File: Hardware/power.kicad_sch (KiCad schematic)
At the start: 16 parts, among them U1 TPS7A20L_1V2, U4 TPS7A20L_2V2, U6 TPS7A20L_3V3, U7 ICE40UL1K-CM36AI

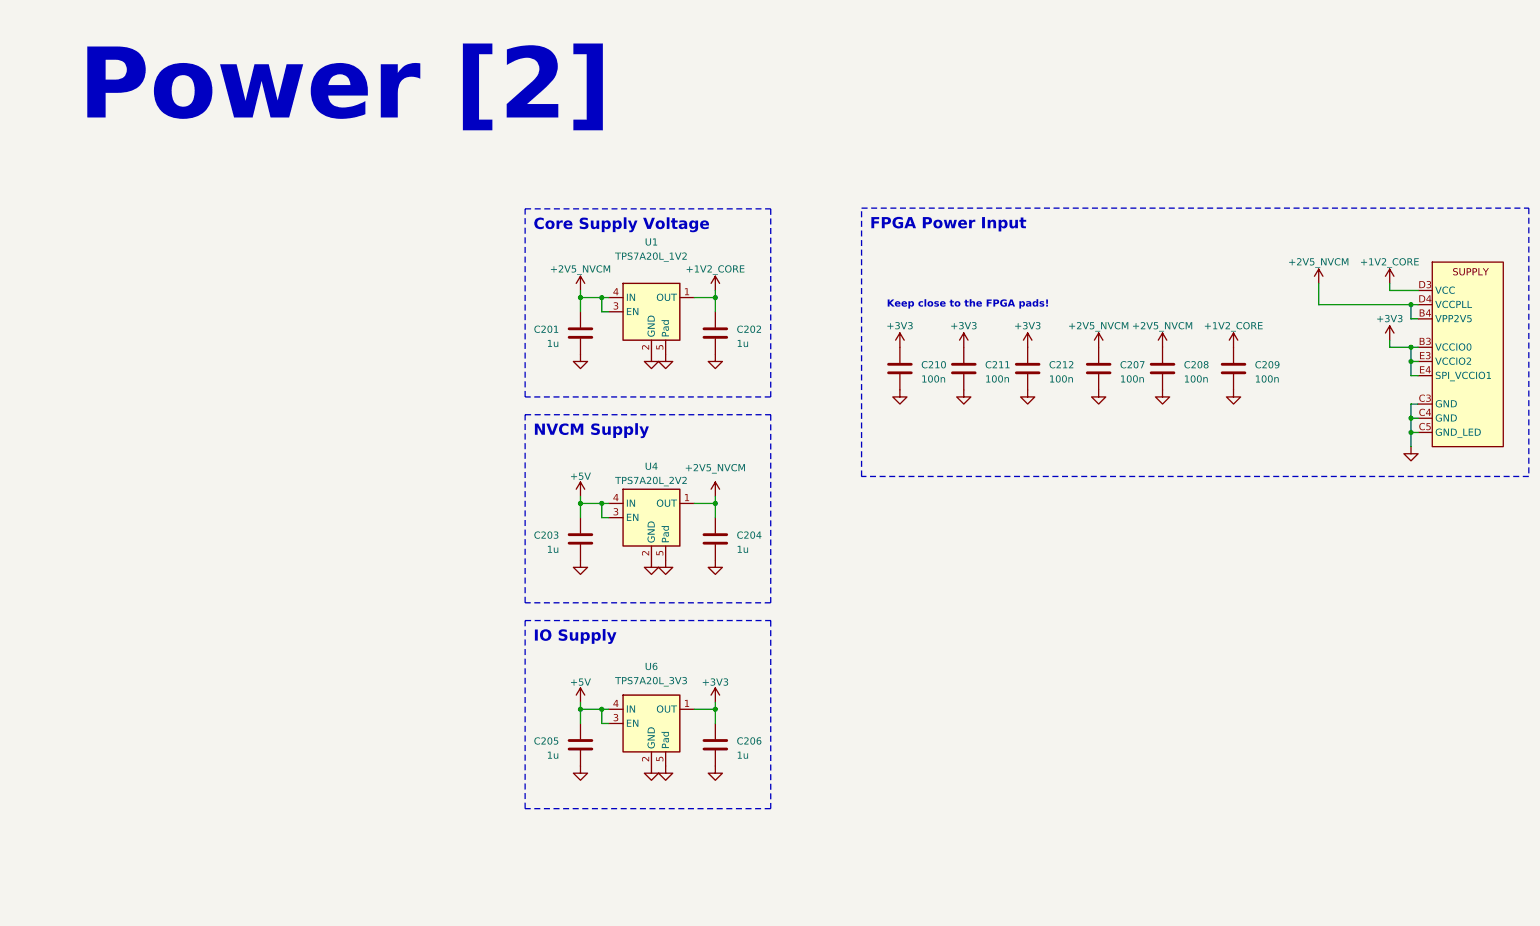
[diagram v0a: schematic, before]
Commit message: Added schematic sections and advanced the design. Advanced the development of Verilog code, for TinyFPGA bringup (however, still not working). Cosmetic changes in README.
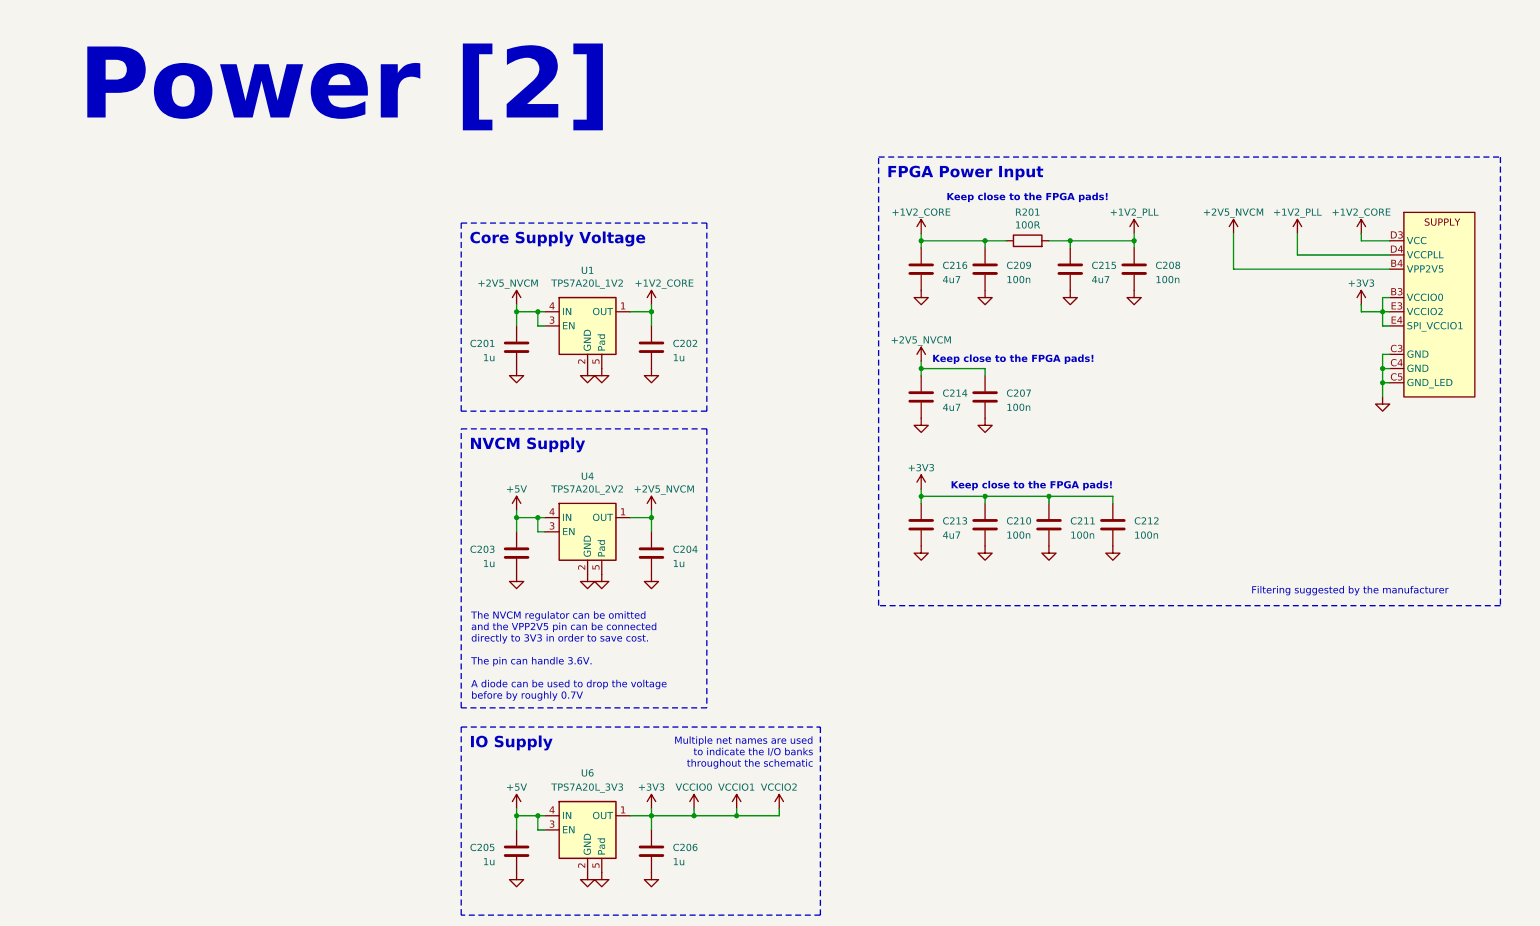
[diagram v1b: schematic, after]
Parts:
- added C213, C214, C215, C216: 4u7, symbol Device:C
- added R201: 100R, symbol Device:R
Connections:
- net +1V2_CORE: now also C216.1, R201.1
- net +2V5_NVCM: now also C214.1; no longer C208.1, U7.D4 (VCCPLL)
- net +3V3: now also C213.1
- net GND: now also C213.2, C214.2, C215.2, C216.2
- new net +1V2_PLL: C208.1, C215.1, R201.2, U7.D4 (VCCPLL)
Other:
- note added: "Filtering suggested by the manufacturer"
- note added: "Multiple net names are used to indicate the I/O banks throughout the schematic"
- note added: "The NVCM regulator can be omitted and the VPP2V5 pin can be connected directly to 3V3 in order to save cost. The pin can handle 3.6V. A diode can be used to drop the voltage before by roughly 0.7V"
- moved on the sheet: C201, C202, C203, C204, C205, C206, C207, C208, C209, C210, C211, C212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

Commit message: Finished the schematic design.
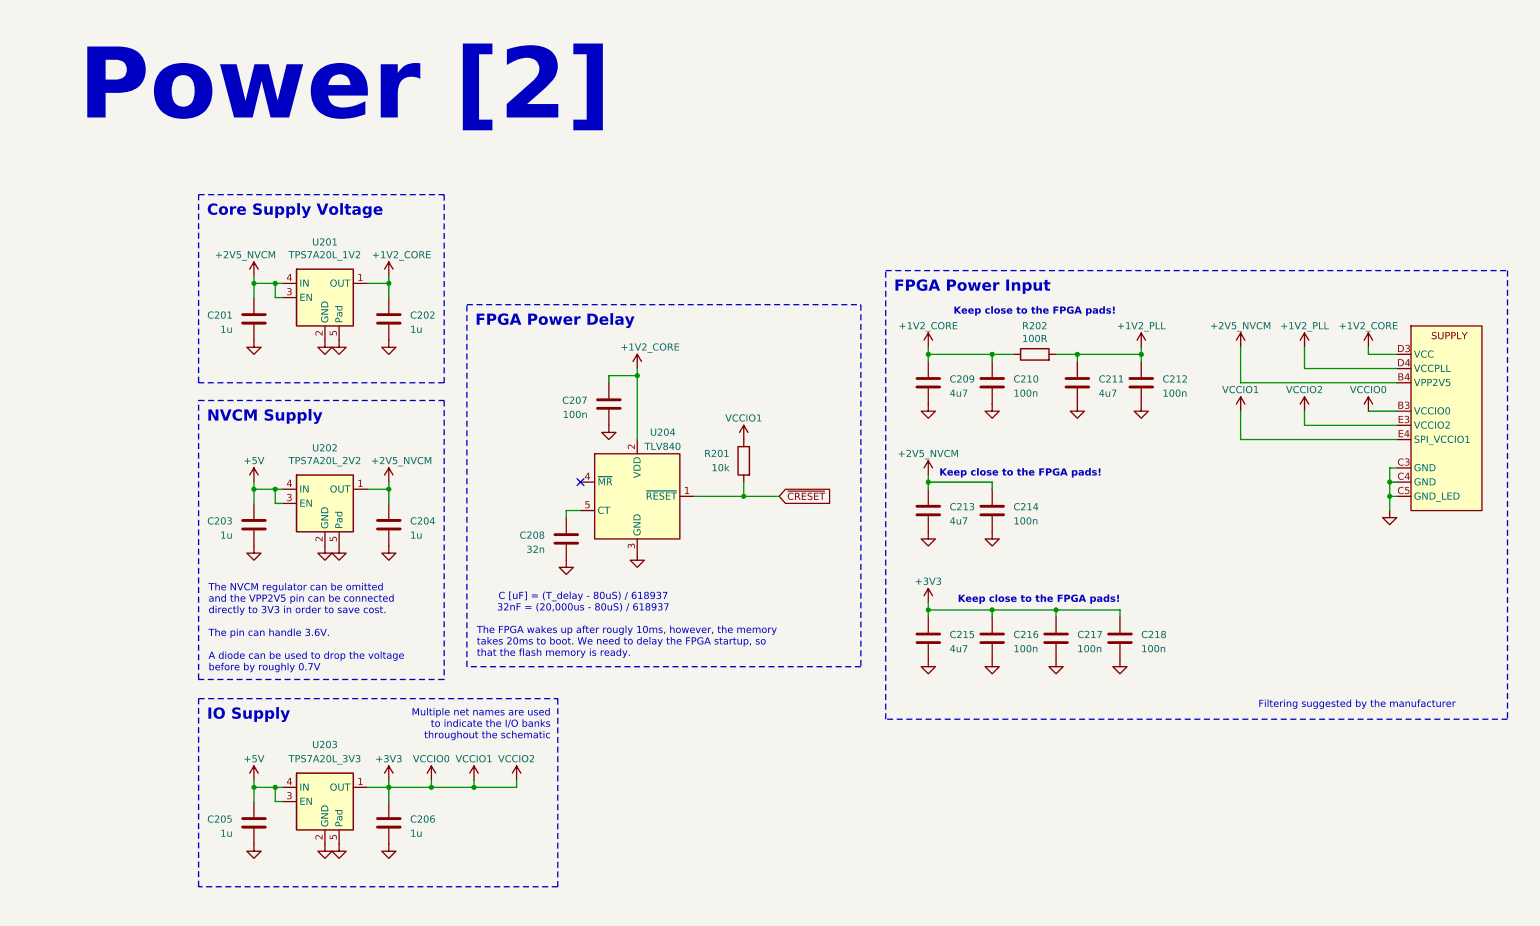
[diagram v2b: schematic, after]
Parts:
- added C207: 100n, Capacitor_SMD:C_0402_1005Metric, symbol Device:C
- added C208: 32n, Capacitor_SMD:C_0402_1005Metric, symbol Device:C
- added R201: 10k, symbol Device:R
- added U204: TLV840, Package_TO_SOT_SMD:SOT-23-5, symbol Custom_VoxLink_Symbols:TLV840
- renumbered C216 to C209, C209 to C210, C215 to C211, C208 to C212, C214 to C213, C207 to C214, C213 to C215, C210 to C216, C211 to C217, C212 to C218, R201 to R202, U1 to U201, U4 to U202, U6 to U203, U7 to U205
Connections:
- net +1V2_CORE: now also C207.1, U204.2 (VDD)
- net +3V3: now also R201.1
- net GND: now also C207.2, C208.2, U204.3 (GND)
- new net: C208.1, U204.5 (CT)
- new net ~{CRESET}: R201.2, U204.1 (~{RESET})
- no-connect marks 0 -> 1
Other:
- note added: "C [uF] = (T_delay - 80uS) / 618937 32nF = (20,000us - 80uS) / 618937"
- note added: "The FPGA wakes up after rougly 10ms, however, the memory takes 20ms to boot. We need to delay the FPGA startup, so that the flash memory is ready."
- moved on the sheet: C201, C202, C203, C204, C205, C206, C209, C210, C211, C212, C213, C214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
